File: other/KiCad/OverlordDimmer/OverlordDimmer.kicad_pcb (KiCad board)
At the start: 2 copper layers, 155.1 x 86.1 mm, 267 parts, among them J1 1757310, J2 1757310, J3 Conn_01x12_Pin, Q1 2N3904, Q10 IRF740, Q11 2N3906, Q12 IRF740, Q13 2N3904, Q14 IRF740, Q15 2N3906, Q16 IRF740, Q17 2N3904, Q18 IRF740, Q19 2N3906, Q2 IRF740, Q20 IRF740, Q21 2N3904, Q22 IRF740, Q23 2N3906, Q24 IRF740, Q25 2N3904, Q26 IRF740, Q27 2N3906, Q28 IRF740, Q29 2N3904, Q3 2N3906, Q30 IRF740, Q31 2N3906, Q32 IRF740, Q33 2N3904, Q34 IRF740, Q35 2N3906, Q36 IRF740, Q37 2N3904, Q38 IRF740, Q39 2N3906, Q4 IRF740, Q40 IRF740, Q41 BC817, Q42 2SC4061KT146N, Q43 2SC4061KT146N, Q5 2N3904, Q6 IRF740, Q7 2N3906, Q8 IRF740, Q9 2N3904, U1 4N25, U10 4N25, U11 SN65HVD230, U2 4N25, U3 4N25, U4 4N25, U5 4N25, U6 4N25, U7 4N25, U8 4N25, U9 4N25

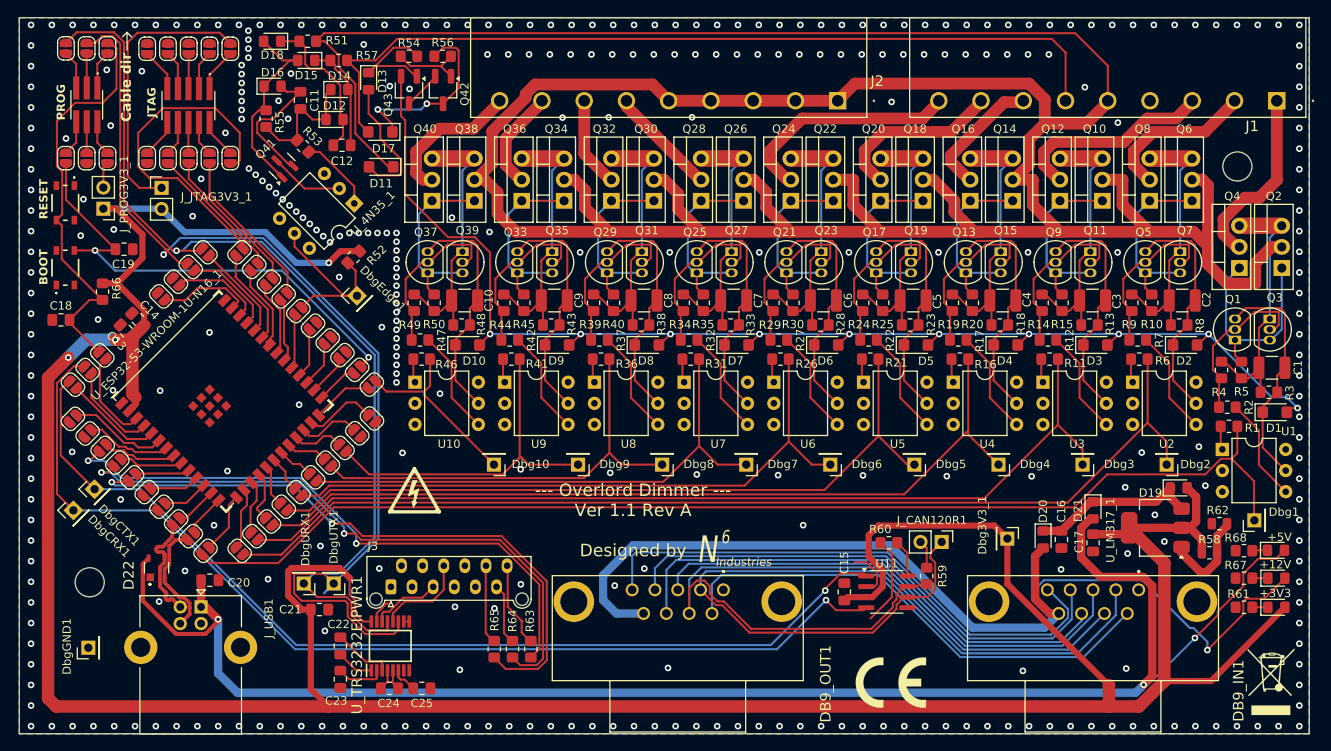
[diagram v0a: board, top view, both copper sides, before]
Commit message: sent to production with fixes
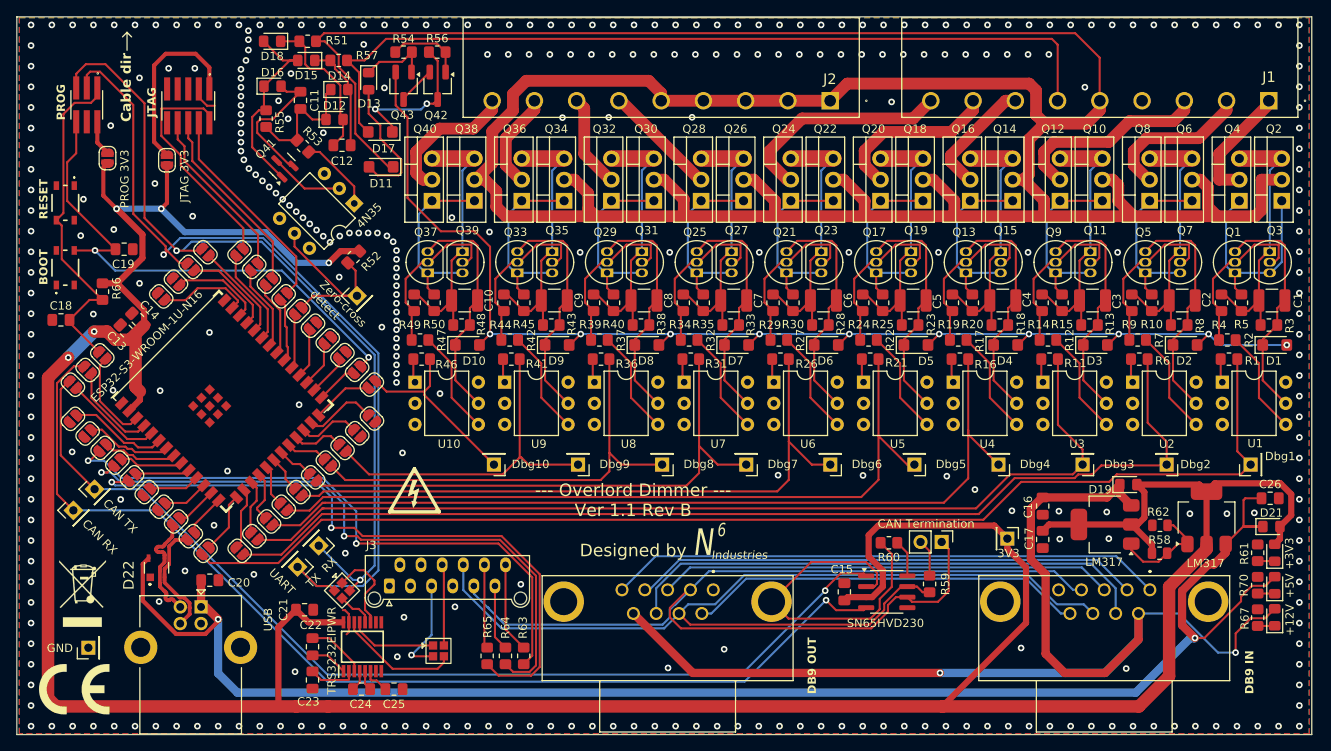
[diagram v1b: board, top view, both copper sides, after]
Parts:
- removed D20: 1N4148, Diode_SMD:D_0805_2012Metric_Pad1.15x1.40mm_HandSolder
- removed H1, H2: MountingHole, MountingHole:MountingHole_3.5mm
- removed JP38, JP39, JP40, JP42, JP43, JP44, JP45, JP46, JP47, JP48, JP50, JP51, JP52, JP53: SolderJumper_2_Open, Jumper:SolderJumper-2_P1.3mm_Open_RoundedPad1.0x1.5mm
- removed J_JTAG1: FTSH-105-01-S-DV-K, OverlordCommon:FTSH-105-XX-YYY-DV-K
- removed J_JTAG3V3_1, J_PROG3V3_1: Conn_01x02_Pin, Connector_PinHeader_2.54mm:PinHeader_1x02_P2.54mm_Vertical
- removed R68: 147, Resistor_SMD:R_0805_2012Metric_Pad1.20x1.40mm_HandSolder
- added C26: 1uF, Capacitor_SMD:C_0805_2012Metric_Pad1.18x1.45mm_HandSolder, F.Cu at (175.9, 83.3)
- added J4: Conn_01x04_Pin, OverlordCommon:Solder_select_2x2, F.Cu at (75.9, 101.7)
- added J5: Conn_01x04_Pin, OverlordCommon:Solder_select_2x2, F.Cu at (64.3, 94.5)
- added J_JTAG2: FTSH-105-01-S-DV-K, OverlordCommon:FTSH-105-XX-YYY-DV-K, F.Cu at (45.8, 36.2)
- added R70: 147, Resistor_SMD:R_0805_2012Metric_Pad1.20x1.40mm_HandSolder, F.Cu at (174.4, 93.8)
- added U_LM317_2: LM317_SOT-223, Package_TO_SOT_SMD:SOT-223-3_TabPin2, F.Cu at (168.2, 85.7)
- moved SYM3 143.3 mm to (33.1, 94.8)
- moved SYM4 98.2 mm to (32.1, 106.3)
- moved D21 21.5 mm to (176.1, 86.8), turned to 0 degrees
- moved R1 8.08 mm to (170.9, 66.6)
- moved R2 8.08 mm to (170.8, 64.3)
- moved C1 8.08 mm to (176.1, 59.6)
- moved Q1 8.08 mm to (171.7, 56.2)
- moved Q2 8.08 mm to (177.3, 47.6)
- moved Q4 8.08 mm to (172.2, 47.6)
- moved D1 8.08 mm to (176.4, 64.9)
- moved Q3 8.08 mm to (175.8, 53.7)
- moved R3 8.08 mm to (175.8, 62.5)
- moved R4 8.08 mm to (170.1, 59.8)
- moved R5 8.08 mm to (172.4, 59.8)
- moved U1 8.08 mm to (170.2, 69.4)
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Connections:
- net Net-(U_LM317_1-ADJ) renamed V_ADJ
- C16 pad 1: Net-(D19-K) -> +12V
- D19 pad 1: Net-(D19-K) -> +12V
- D21 pad 1: Net-(D19-K) -> +5V
- D21 pad 2: +5V -> +3.3V
- DB9_IN1 pad 1: GND -> MB2_H
- DB9_IN1 pad 2: CAN_L -> MB2_L
- DB9_IN1 pad 4: MB2_L -> CAN_L
- DB9_IN1 pad 5: MB2_H -> GND
- DB9_IN1 pad 6: MB1_L -> +12V
- DB9_IN1 pad 7: CAN_H -> MB1_H
- DB9_IN1 pad 8: MB1_H -> CAN_H
- DB9_IN1 pad 9: +12V -> MB1_L
- J3 pad 8: unconnected-(J3-Pin_8-Pad8) -> CAN_H
- J3 pad 9: unconnected-(J3-Pin_9-Pad9) -> CAN_L
- JP41 pad 2: JTAG_TCK -> +3.3V
- JP49 pad 2: Net-(JP49-B) -> +3.3V
- J_PROG1 pad 1: Net-(JP48-B) -> ESP_EN
- J_PROG1 pad 3: Net-(JP50-B) -> UART_TX_0
- J_PROG1 pad 4: Net-(JP51-A) -> GND
- J_PROG1 pad 5: Net-(JP52-B) -> UART_RX_0
- J_PROG1 pad 6: Net-(JP53-A) -> ESP_IO0
- U_LM317_1 pad 3: Net-(D19-K) -> +12V
- U_TRS3232EIPWR1 pad 11: UART_TX_0 -> Net-(J5-Pin_1)
- U_TRS3232EIPWR1 pad 12: RS232_RX -> Net-(J5-Pin_2)
- U_TRS3232EIPWR1 pad 13: UART_RX_0 -> Net-(J4-Pin_1)
- U_TRS3232EIPWR1 pad 14: RS232_TX -> Net-(J4-Pin_2)
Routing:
- net Net-(JP38-A): track 34.1 -> 0.00 mm
- net L: track 408.0 -> 377.1 mm
- net GND: track 20.3 -> 48.2 mm, vias 341 -> 337
- net CAN_L: track 100.1 -> 127.7 mm
- net Net-(D19-K): track 20.5 -> 0.00 mm
- net CAN_H: track 98.3 -> 118.5 mm
- net UART_TX_0: track 125.7 -> 107.5 mm
- net Net-(JP41-A): track 4.16 -> 21.9 mm
- net +12V: track 123.2 -> 140.4 mm, vias 1 -> 2
- net UART_RX_0: track 116.0 -> 100.9 mm, vias 1 -> 2
- net Net-(J4-Pin_2): track 0.00 -> 14.7 mm
- net MB1_L: track 60.2 -> 47.7 mm
- net JTAG_TMS: track 40.4 -> 28.0 mm
- net Net-(J5-Pin_1): track 0.00 -> 10.8 mm
- net Net-(J4-Pin_1): track 0.00 -> 10.6 mm
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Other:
- board size 155.1 x 86.1 mm -> 155.7 x 86.3 mm
- board text added: "--- Overlord Dimmer --- Ver 1.1 Rev B Designed by"
- board text added: "3V3"
- board text added: "4N35"
- board text added: "CAN RX"
- board text added: "CAN TX"
- board text added: "CAN Termination"
- board text added: "DB9 IN"
- board text added: "DB9 OUT"
- board text added: "ESP32-S3-WROOM-1U-N16"
- board text added: "GND"
- board text added: "JTAG 3V3"
- board text added: "LM317"
- board text added: "PROG 3V3"
- board text added: "SN65HVD230"
- board text added: "TRS3232EIPWR"
- board text added: "TX RX"
- board text added: "UART"
- board text added: "USB"
- board text added: "Zero-cross detect"
- board text removed: "--- Overlord Dimmer --- Ver 1.1 Rev A Designed by"
